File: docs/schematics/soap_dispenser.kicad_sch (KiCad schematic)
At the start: 6 parts, among them J1 Infrared Obstacle Sensor, M1 R280 Diaphragm Pump, Q1 1RLZ44N MOSFET

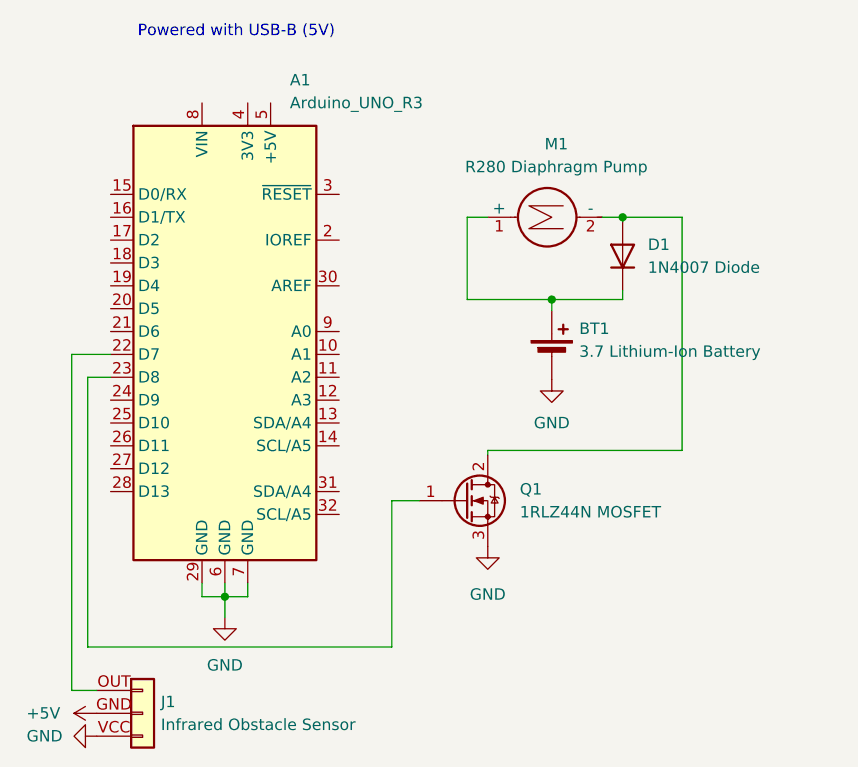
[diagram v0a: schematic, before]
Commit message: fixed schematics
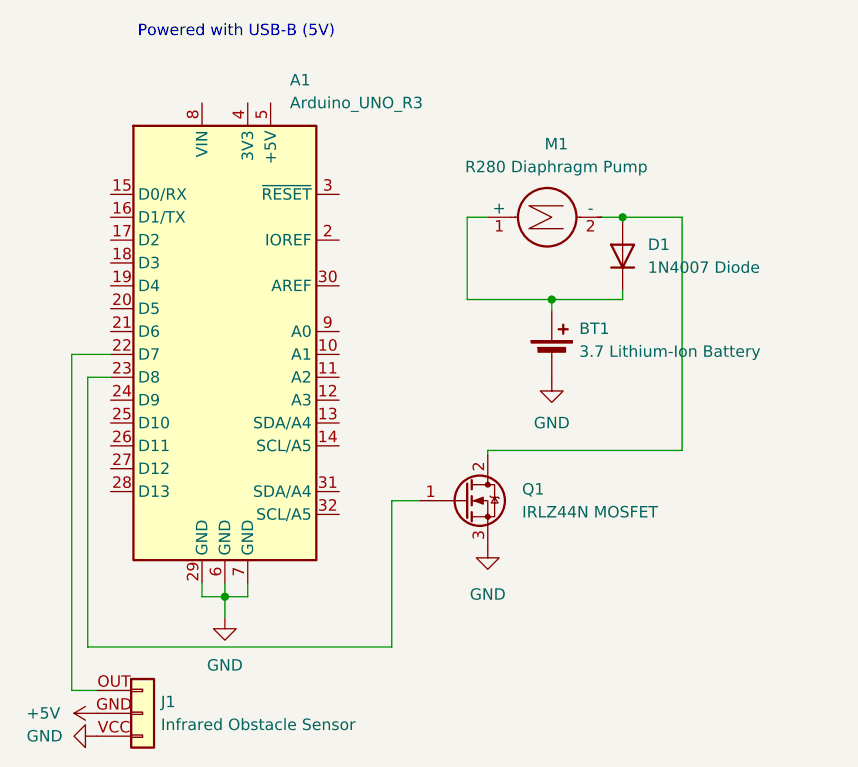
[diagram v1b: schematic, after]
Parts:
- Q1: value 1RLZ44N MOSFET -> IRLZ44N MOSFET
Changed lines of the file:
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@@
 		)
 		(instances
-			(project "self_charge"
+			(project "soap_dispenser"
 				(path "/62ccd462-d44e-41d8-96cb-b7e5dd7d1810"
 					(reference "#PWR02")
@@
 		)
 		(instances
-			(project "self_charge"
+			(project "soap_dispenser"
 				(path "/62ccd462-d44e-41d8-96cb-b7e5dd7d1810"
 					(reference "#PWR03")
@@
 		)
 		(instances
-			(project "self_charge"
+			(project "soap_dispenser"
 				(path "/62ccd462-d44e-41d8-96cb-b7e5dd7d1810"
 					(reference "A1")
@@
 		)
 		(instances
-			(project "self_charge"
+			(project "soap_dispenser"
 				(path "/62ccd462-d44e-41d8-96cb-b7e5dd7d1810"
 					(reference "BT1")
@@
 		)
 		(instances
-			(project "self_charge"
+			(project "soap_dispenser"
 				(path "/62ccd462-d44e-41d8-96cb-b7e5dd7d1810"
 					(reference "J1")
@@
 		)
 		(instances
-			(project "self_charge"
+			(project "soap_dispenser"
 				(path "/62ccd462-d44e-41d8-96cb-b7e5dd7d1810"
 					(reference "M1")
@@
 		(fields_autoplaced yes)
 		(property "Reference" "Q1"
-			(at 147.066 117.8559 0)
-			(show_name no)
-			(do_not_autoplace no)
-			(effects
-				(font
-					(size 1.27 1.27)
-				)
-				(justify left)
-			)
-		)
-		(property "Value" "1RLZ44N MOSFET"
-			(at 147.066 120.3959 0)
+			(at 147.32 117.8559 0)
+			(show_name no)
+			(do_not_autoplace no)
+			(effects
+				(font
+					(size 1.27 1.27)
+				)
+				(justify left)
+			)
+		)
+		(property "Value" "IRLZ44N MOSFET"
+			(at 147.32 120.3959 0)
 			(show_name no)
 			(do_not_autoplace no)
@@
 		)
 		(instances
-			(project "self_charge"
+			(project "soap_dispenser"
 				(path "/62ccd462-d44e-41d8-96cb-b7e5dd7d1810"
 					(reference "Q1")
@@
 		)
 		(instances
-			(project "self_charge"
+			(project "soap_dispenser"
 				(path "/62ccd462-d44e-41d8-96cb-b7e5dd7d1810"
 					(reference "#PWR01")
@@
 		)
 		(instances
-			(project "self_charge"
+			(project "soap_dispenser"
 				(path "/62ccd462-d44e-41d8-96cb-b7e5dd7d1810"
 					(reference "#PWR04")
@@
 		)
 		(instances
-			(project "self_charge"
+			(project "soap_dispenser"
 				(path "/62ccd462-d44e-41d8-96cb-b7e5dd7d1810"
 					(reference "#PWR06")
@@
 		)
 		(instances
-			(project "self_charge"
+			(project "soap_dispenser"
 				(path "/62ccd462-d44e-41d8-96cb-b7e5dd7d1810"
 					(reference "D1")
